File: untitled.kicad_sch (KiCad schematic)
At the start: 0 parts

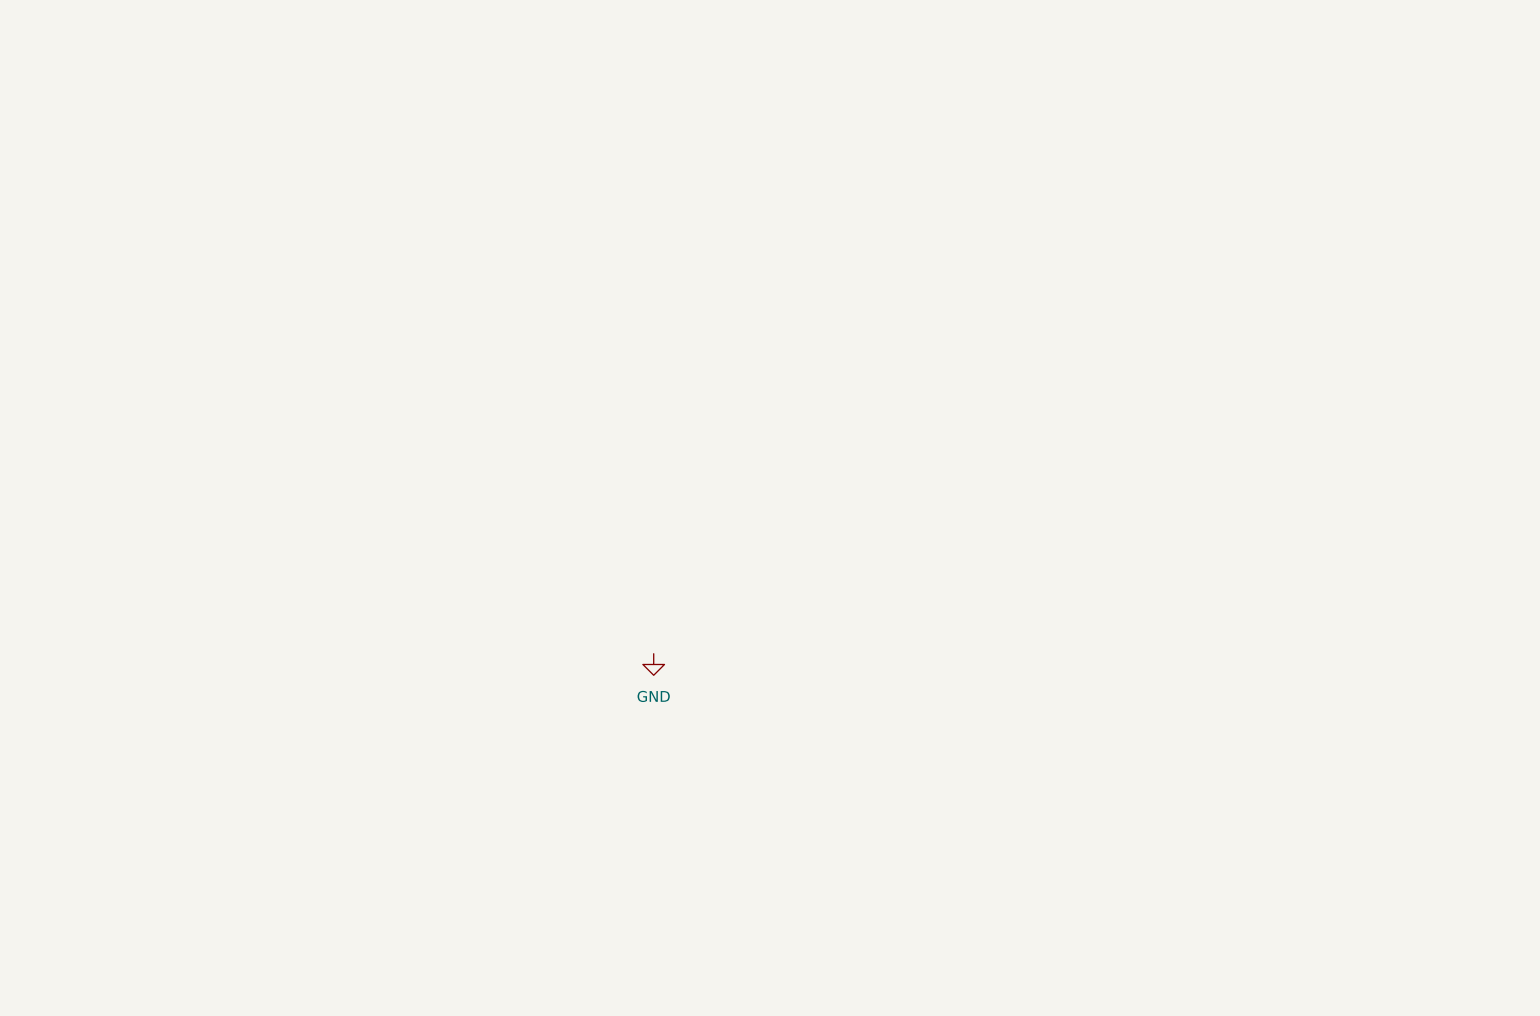
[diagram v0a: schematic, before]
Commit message: VGA design
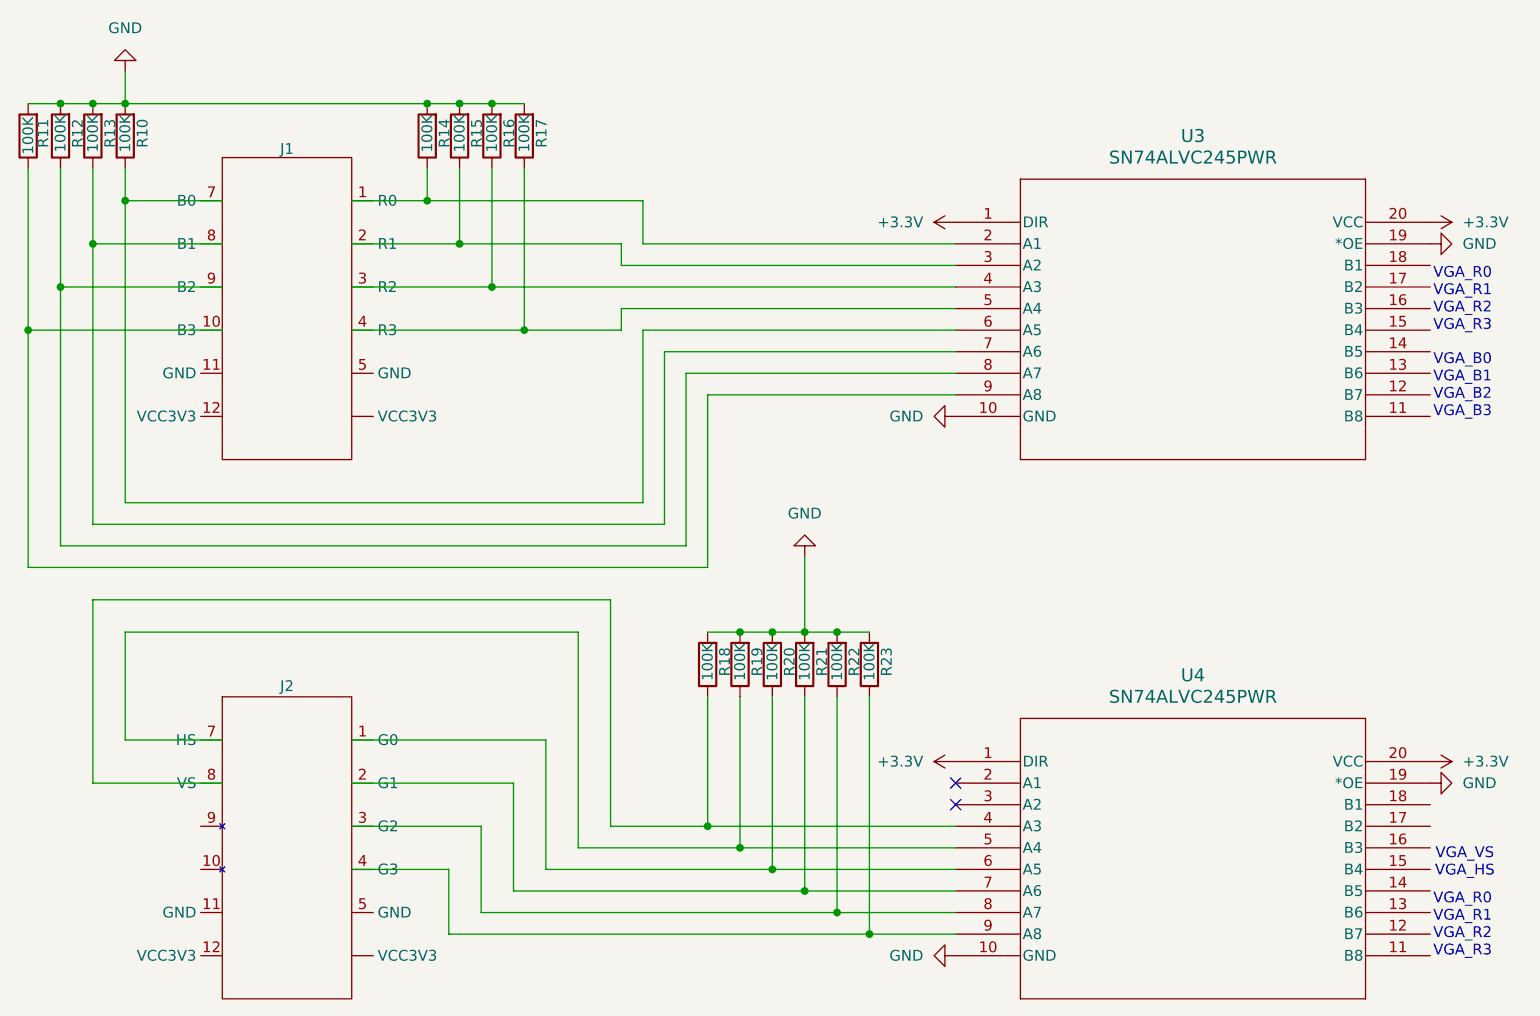
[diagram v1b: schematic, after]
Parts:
- added J1: ~, symbol PMod:PMod j1
- added J2: ~, symbol PMod:PMod_j2
- added R10, R11, R12, R13, R14, R15, R16, R17, R18, R19, R20, R21, R22, R23: 100K, symbol Device:R
- added U3, U4: SN74ALVC245PWR, PW20, symbol 2025-09-12_09-11-34:SN74ALVC245PWR
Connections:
- net GND: now also R10.2, R11.2, R12.2, R13.2, R14.2, R15.2, R16.2, R17.2, R18.2, R19.2, R20.2, R21.2, R22.2, R23.2, U3.10 (GND), U3.19 (*OE), U4.10 (GND), U4.19 (*OE)
- new net: J1.7 (B0), R10.1, U3.6 (A5)
- new net: J2.2 (G1), R21.1, U4.7 (A6)
- new net: J1.1 (R0), R14.1, U3.2 (A1)
- new net: J1.10 (B3), R11.1, U3.9 (A8)
- new net: J1.2 (R1), R15.1, U3.3 (A2)
- new net: J1.3 (R2), R16.1, U3.4 (A3)
- new net: J1.4 (R3), R17.1, U3.5 (A4)
- new net: J1.8 (B1), R13.1, U3.7 (A6)
- new net: J1.9 (B2), R12.1, U3.8 (A7)
- new net: J2.3 (G2), R22.1, U4.8 (A7)
- new net: J2.8 (VS), R18.1, U4.4 (A3)
- new net: J2.4 (G3), R23.1, U4.9 (A8)
- new net: J2.1 (G0), R20.1, U4.6 (A5)
- new net: J2.7 (HS), R19.1, U4.5 (A4)
- new net +3.3V: U3.1 (DIR), U3.20 (VCC), U4.1 (DIR), U4.20 (VCC)
- no-connect marks 0 -> 2
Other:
- note added: "VGA_B0 VGA_B1 VGA_B2 VGA_B3"
- note added: "VGA_R0 VGA_R1 VGA_R2 VGA_R3"
- note added: "VGA_VS VGA_HS"
